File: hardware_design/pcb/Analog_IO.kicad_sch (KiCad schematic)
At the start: 37 parts, among them Q2 MMBT3904, Q3 MMBT3904, U3 TL072CD, U4 TL072CD

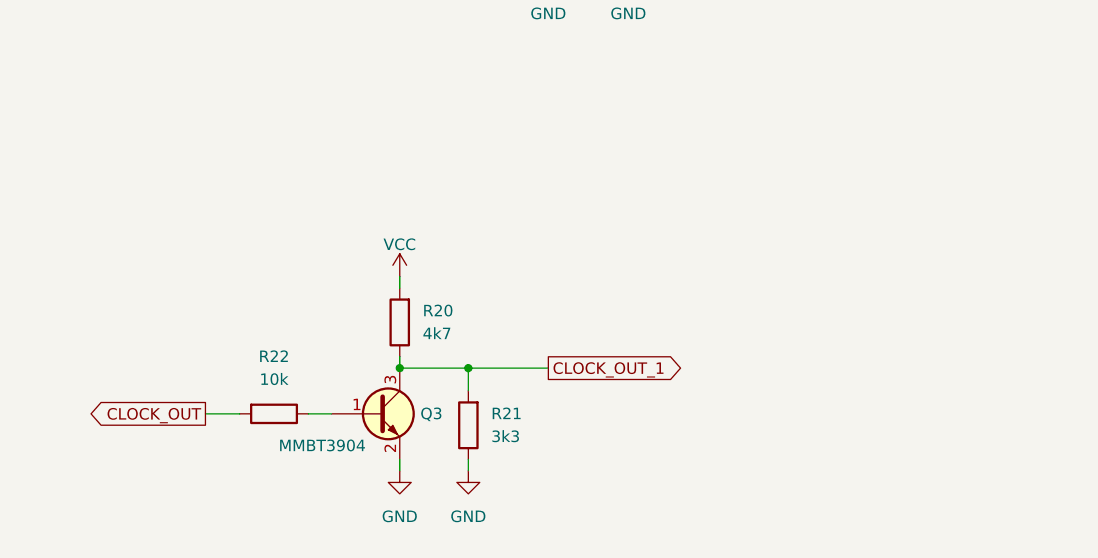
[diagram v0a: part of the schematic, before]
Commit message: Rev 2 schematic & circuit board
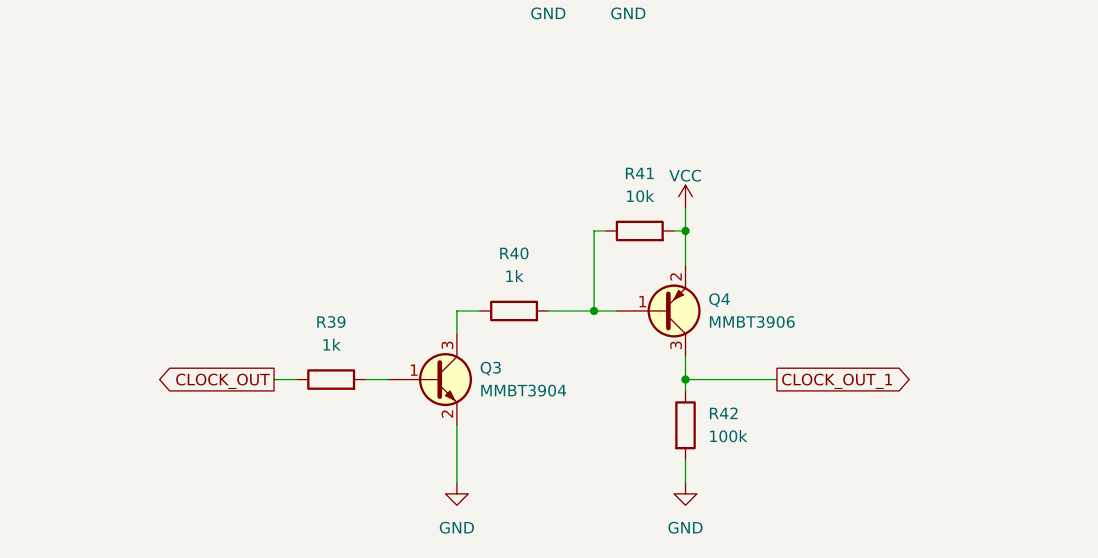
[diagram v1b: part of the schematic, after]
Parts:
- removed R20: 4k7, Resistor_SMD_AKL:R_0603_1608Metric_Pad1.05x0.95mm_HandSolder, symbol Resistor_AKL:R_0603
- removed R21: 3k3, Resistor_SMD_AKL:R_0603_1608Metric_Pad1.05x0.95mm_HandSolder, symbol Resistor_AKL:R_0603
- removed R22: 10k, Resistor_SMD_AKL:R_0603_1608Metric_Pad1.05x0.95mm_HandSolder, symbol Resistor_AKL:R_0603
- added Q4: MMBT3906, Package_TO_SOT_SMD_AKL:SOT-23, symbol Transistor_BJT_AKL:MMBT3906
- added R39, R40: 1k, Resistor_SMD_AKL:R_0603_1608Metric_Pad1.05x0.95mm_HandSolder, symbol Resistor_AKL:R_0603
- added R41: 10k, Resistor_SMD_AKL:R_0603_1608Metric_Pad1.05x0.95mm_HandSolder, symbol Resistor_AKL:R_0603
- added R42: 100k, Resistor_SMD_AKL:R_0603_1608Metric_Pad1.05x0.95mm_HandSolder, symbol Resistor_AKL:R_0603
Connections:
- net CLOCK_OUT: now also R39.1
- net CLOCK_OUT_1: now also Q4.3 (C), R42.1; no longer Q3.3 (C)
- net GND: now also R42.2
- net VCC: now also Q4.2 (E), R41.2
- net at Q3.1 (B): now also R39.2
- new net: Q4.1 (B), R40.2, R41.1
- new net: Q3.3 (C), R40.1
